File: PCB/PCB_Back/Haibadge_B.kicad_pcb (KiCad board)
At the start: 2 copper layers, 80 x 80 mm, 69 parts, among them J1 Sensor connector, J2 USB_C_Receptacle_USB2.0, J3 Lipo connector, Q1 UMH3N, Q2 PMOS, SW1 SW_Push_Dual, U1 ESP-12E, U2 CH340C, U3 MCP73831-2-OT, U4 MCP1700x-330xxTT, U6 BME680

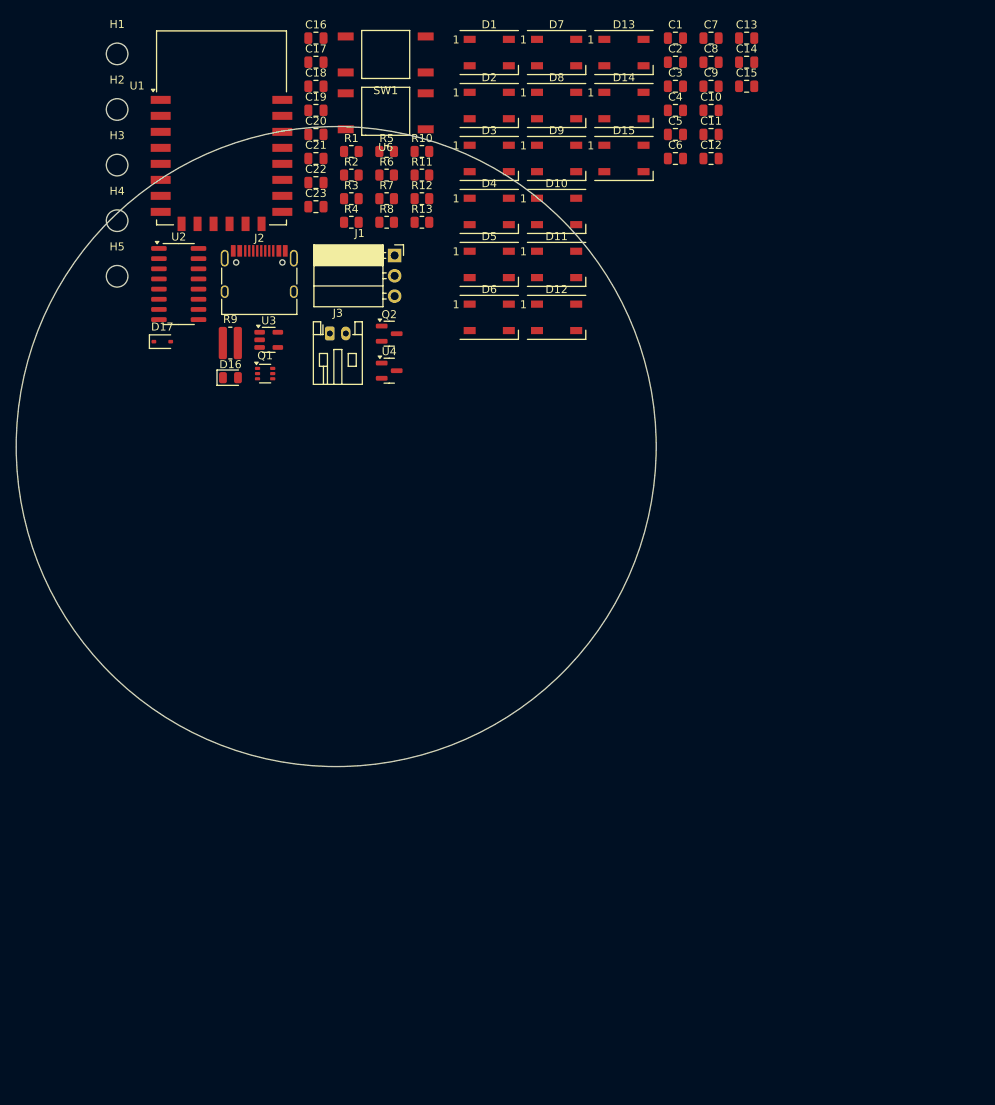
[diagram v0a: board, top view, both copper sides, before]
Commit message: Layout, Routing, Stuff
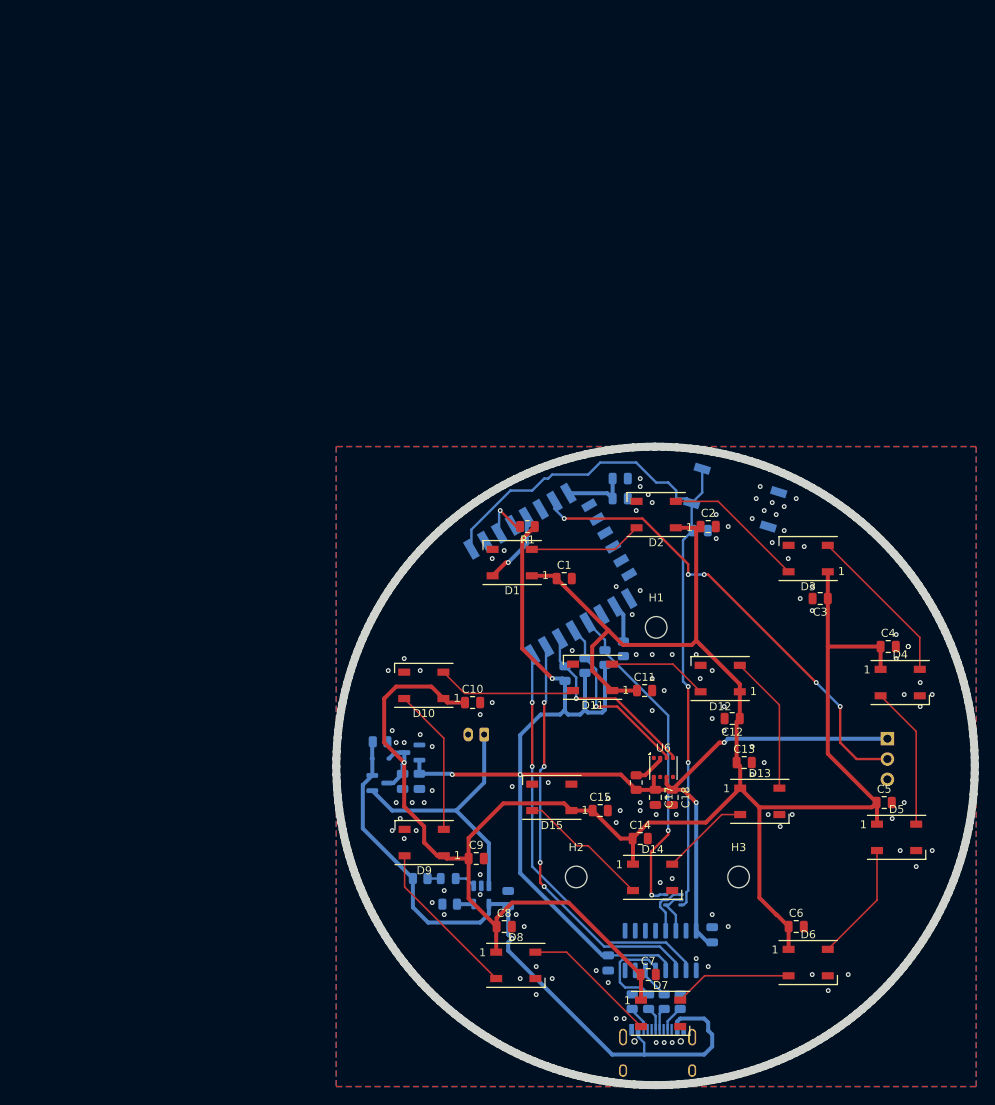
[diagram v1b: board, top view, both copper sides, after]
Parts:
- removed H4, H5: MountingHole, MountingHole:MountingHole_2.7mm_M2.5
- added ? (x5): , Graphics, F.Cu at (100.0, 100.0)
- added ? (x3): , Graphics, F.Cu at (200.0, 47.5)
- added C24: 100nF, Capacitor_SMD:C_0805_2012Metric, B.Cu at (134.0, 164.6)
- added C25: 100nF, Capacitor_SMD:C_0805_2012Metric, B.Cu at (147.0, 161.0)
- C16, C19, C20, C21, C22, C23, D16, D17, J1, J2, J3, Q1, Q2, R10, R11, R12, R13, R2, R4, R5, R6, R7, R8, SW1, U1, U2, U3, U4: moved to B.Cu
- R9: footprint Resistor_SMD:R_0815_2038Metric -> Resistor_SMD:R_0805_2012Metric; moved to B.Cu
- U6: footprint KH-6X6X6H-STM:KH-6X6X6H-STM -> Package_LGA:Bosch_LGA-8_3x3mm_P0.8mm_ClockwisePinNumbering
- moved D7 120.8 mm to (140.6, 170.8)
- moved H3 118.1 mm to (150.3, 153.8)
- moved C7 117.3 mm to (139.0, 166.0)
- moved R5 112.4 mm to (143.0, 169.4), turned to 90 degrees
- moved H2 111.8 mm to (130.0, 153.8)
- moved C8 111.1 mm to (121.0, 160.0)
- moved J2 109.4 mm to (140.2, 176.9), turned to 180 degrees
- moved R6 107.8 mm to (137.0, 169.4), turned to -90 degrees
- moved D8 107.6 mm to (122.5, 164.8)
- moved R7 105.6 mm to (139.1, 169.4), turned to 90 degrees
- moved R8 103.4 mm to (141.0, 169.4), turned to -90 degrees
- moved U2 102.8 mm to (140.6, 163.0), turned to 90 degrees
- moved C17 101.2 mm to (139.9, 143.8), turned to -90 degrees
- moved C9 100.9 mm to (117.5, 151.5)
- moved C18 99.4 mm to (142.0, 143.8), turned to -90 degrees
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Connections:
- D11 pad 4: Net-(D11-DIN) -> Net-(D10-DOUT)
- D12 pad 4: Net-(D12-DIN) -> Net-(D11-DOUT)
- D13 pad 4: Net-(D10-DOUT) -> Net-(D12-DOUT)
- D14 pad 4: Net-(D11-DOUT) -> Net-(D13-DOUT)
- D15 pad 4: Net-(D12-DOUT) -> Net-(D14-DOUT)
- D2 pad 4: Net-(D13-DOUT) -> Net-(D1-DOUT)
- D3 pad 4: Net-(D14-DOUT) -> Net-(D2-DOUT)
- D4 pad 4: Net-(D1-DOUT) -> Net-(D3-DOUT)
- D5 pad 4: Net-(D2-DOUT) -> Net-(D4-DOUT)
- D6 pad 4: Net-(D3-DOUT) -> Net-(D5-DOUT)
- D7 pad 2: Net-(D10-DIN) -> Net-(D7-DOUT)
- D7 pad 4: Net-(D4-DOUT) -> Net-(D6-DOUT)
- D8 pad 2: Net-(D11-DIN) -> Net-(D8-DOUT)
- D8 pad 4: Net-(D5-DOUT) -> Net-(D7-DOUT)
- D9 pad 2: Net-(D12-DIN) -> Net-(D10-DIN)
- D9 pad 4: Net-(D6-DOUT) -> Net-(D8-DOUT)
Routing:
- net VCC: track 0.00 -> 288.0 mm, vias 0 -> 1
- net +3V3: track 0.00 -> 188.4 mm, vias 0 -> 5
- net RST: track 0.00 -> 92.6 mm, vias 0 -> 2
- net +5V: track 0.00 -> 87.4 mm, vias 0 -> 1
- net Sensor: track 0.00 -> 58.9 mm, vias 0 -> 5
- net Net-(U1-GPIO3/RXD): track 0.00 -> 51.9 mm, vias 0 -> 4
- net Net-(U1-GPIO1/TXD): track 0.00 -> 51.7 mm, vias 0 -> 2
- net GPIO0: track 0.00 -> 41.0 mm, vias 0 -> 2
- net +BATT: track 0.00 -> 33.6 mm
- net Net-(U1-GPIO5): track 0.00 -> 24.6 mm, vias 0 -> 1
- net Net-(U1-GPIO4): track 0.00 -> 22.3 mm, vias 0 -> 1
- net Net-(D3-DOUT): track 0.00 -> 20.3 mm
- net Net-(D8-DOUT): track 0.00 -> 20.1 mm
- net Net-(D10-DIN): track 0.00 -> 18.4 mm
- net Net-(D4-DOUT): track 0.00 -> 17.9 mm
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- added copper zone on B.Cu, net GND
- added copper zone on F.Cu, net GND
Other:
- board size 80 x 80 mm -> 79.8 x 79.8 mm
- board text added: "${REFERENCE}"
